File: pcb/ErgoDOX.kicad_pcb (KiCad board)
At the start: 2 copper layers, 182.8 x 158.9 mm, 77 parts, among them J1 USB, J2 3.5mm, J3 JMP, J4 JMP, SW0:10 SW0:3, SW0:11 SW0:2, SW0:12 SW0:1, SW0:7 SW0:6, SW0:8 SW0:5, SW0:9 SW0:4, SW1:10 SW1:3, SW1:11 SW1:2, SW1:12 SW1:1, SW1:13 SW1:0, SW1:9 SW1:4, SW2:10 SW2:3, SW2:11 SW2:2, SW2:12 SW2:1, SW2:13 SW2:0, SW2:7 SW2:6, SW2:8 SW2:5, SW2:9 SW2:4, SW3:10 SW3:3, SW3:11 SW3:2, SW3:12 SW3:1, SW3:13 SW3:0, SW3:8 SW3:5, SW3:9 SW3:4, SW4:10 SW4:3, SW4:11 SW4:2, SW4:12 SW4:1, SW4:13 SW4:0, SW4:7 SW4:6, SW4:8 SW4:5, SW4:9 SW4:4, SW5:10 SW5:3, SW5:11 SW5:2, SW5:12 SW5:1, SW5:13 SW5:0, SW5:7 SW5:6, SW5:8 SW5:5, SW5:9 SW5:4, U1 TEENSY2.0, U2 MCP23018

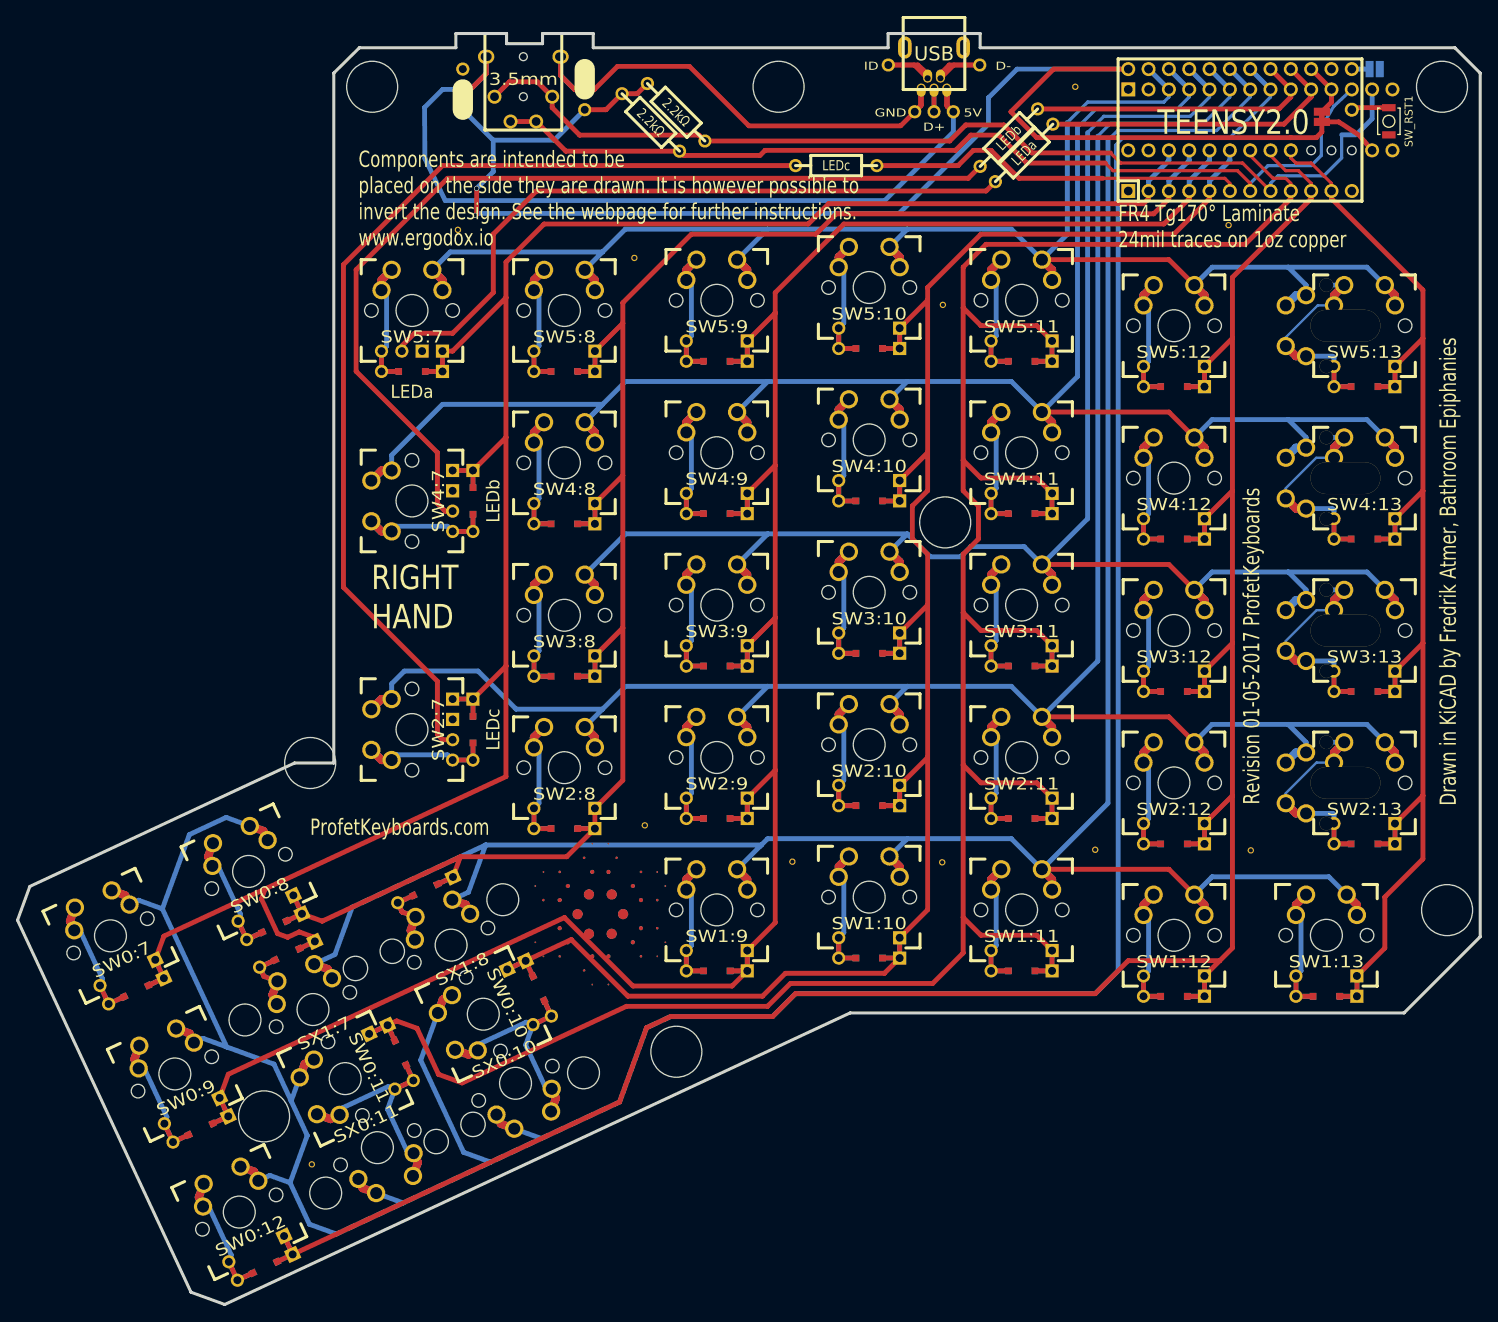
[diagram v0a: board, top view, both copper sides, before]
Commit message: starting routing
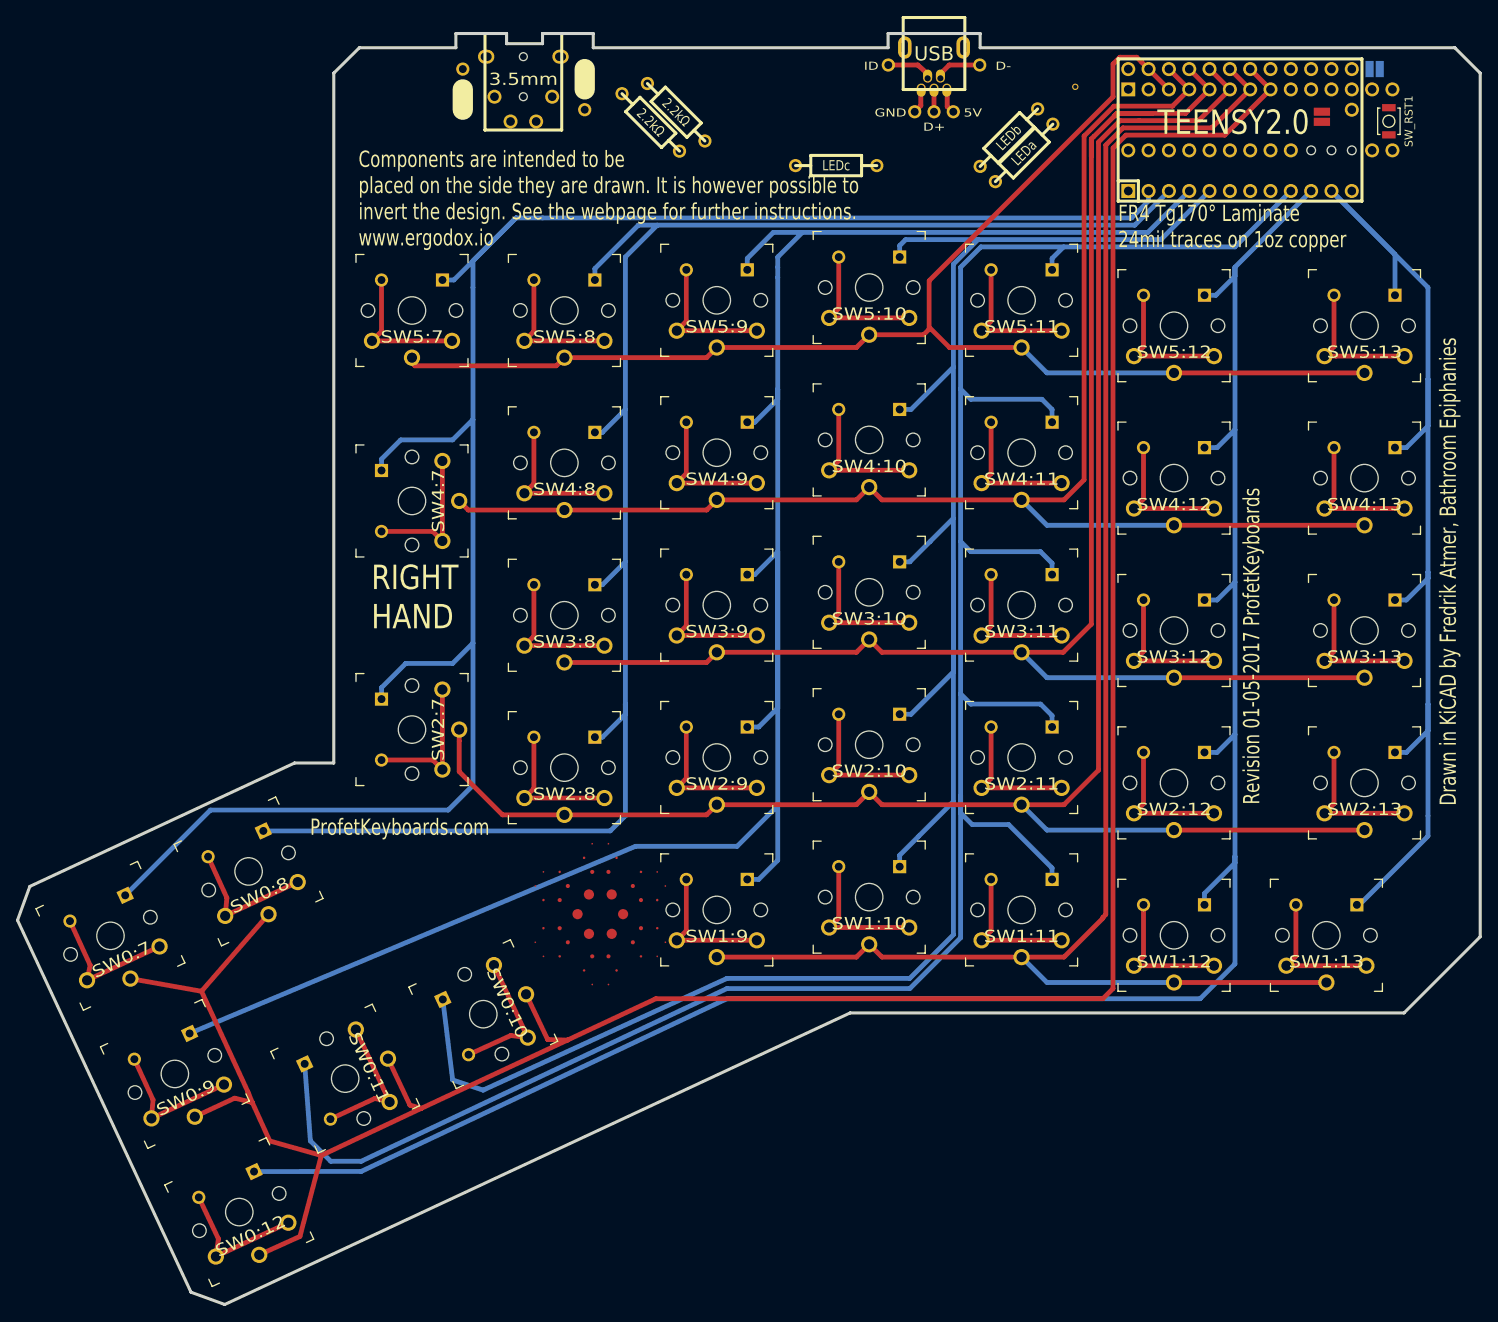
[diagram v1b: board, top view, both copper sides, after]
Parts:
- removed D1:7, D1:8: D, DIODE
- removed H99: MECHANICAL, ErgoDOXmech
- removed LED_A1: LEDa, MX_LED
- removed LED_B1: LEDb, MX_LED
- removed LED_C1: LEDc, MX_LED
- removed S1, S2: STAB200, STAB_PCB940
- removed STAR_2: STAR_BACK, ErgoDOX pcb:STAR
- removed the STITCHING_VIA at (100.2, 58.5)
- removed the STITCHING_VIA at (78.1, 55.0)
- removed the STITCHING_VIA at (138.8, 64.4)
- removed the STITCHING_VIA at (177.2, 132.6)
- removed the STITCHING_VIA at (157.8, 132.5)
- removed the STITCHING_VIA at (138.7, 134.1)
- removed the STITCHING_VIA at (119.9, 134.0)
- removed the STITCHING_VIA at (59.9, 171.8)
- removed the STITCHING_VIA at (101.5, 129.5)
- removed the STITCHING_VIA at (174.5, 54.4)
- removed SX0:10: SX0:3, MX_FLIP
- removed SX0:11: SX0:2, MX_FLIP
- removed SX1:7: SX1:6, MX_FLIP
- removed SX1:8: SX1:5, MX_FLIP
- SW0:10, SW0:11, SW0:12, SW0:7, SW0:8, SW0:9, SW1:10, SW1:11, SW1:12, SW1:13, SW1:9, SW2:10, SW2:11, SW2:12, SW2:7, SW2:8, SW2:9, SW3:10, SW3:11, SW3:12, SW3:8, SW3:9, SW4:10, SW4:11, SW4:12, SW4:7, SW4:8, SW4:9, SW5:10, SW5:11, SW5:12, SW5:7, SW5:8, SW5:9: footprint ErgoDOX pcb:MX_FLIP_DIODE -> switch_footprints:SW_PG1350_reversible
- SW2:13, SW3:13, SW4:13, SW5:13: footprint ErgoDOX pcb:MX_FLIP_XX -> switch_footprints:SW_PG1350_reversible
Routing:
- net VCC: track 204.8 -> 0.00 mm, vias 2 -> 0
- net /SDAM: track 128.3 -> 0.00 mm
- net Net-(LED_C1-Pad1): track 127.4 -> 0.00 mm
- net /SCLM: track 119.7 -> 0.00 mm
- net Net-(LED_B1-Pad1): track 119.1 -> 0.00 mm
- net /ROW1: track 318.2 -> 212.3 mm
- net Net-(J1-Pad1): track 102.6 -> 0.00 mm
- net Net-(LED_A1-Pad1): track 87.6 -> 0.00 mm
- net /ROW0: track 404.2 -> 324.8 mm
- net /ROW4: track 257.4 -> 187.8 mm
- net Net-(J1-Pad5): track 62.3 -> 0.00 mm
- net /ROW2: track 295.3 -> 236.5 mm
- net /ROW5: track 225.1 -> 175.5 mm
- net /LED_C: track 47.6 -> 0.00 mm
- net /LED_A: track 38.2 -> 0.00 mm
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- removed copper zone on B.Cu, net GND
- removed copper zone on F.Cu, net GND
